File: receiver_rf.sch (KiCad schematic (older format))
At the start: 0 parts

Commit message: Added mixer and LNA
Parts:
- added C? (x2): 22pF, symbol Device:C
- added C?: 22uF, symbol Device:C
- added C?: 100pF, symbol Device:C
- added L?: 10nH, symbol Device:L
- added U?: PMA-63GLN+, symbol own:PMA-63GLN+
- added U?: HMC218BMS8GE, symbol own:HMC218BMS8GE
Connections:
- new net: C?.2, U?.2 (RF_IN)
- new net: C?.1, L?.2, U?.8 (RF_OUT/DC_IN)
- new net: C?.2, U?.8 (RF)
- new net +5V: C?.2, C?.2, L?.1
- new net GND: C?.1, C?.1, U?.13 (GND/Paddle), U?.2 (GND), U?.3 (GND), U?.6 (GND), U?.7 (GND)
- new net IF_OUT: U?.5 (IF)
- new net LO_IN: U?.1 (LO)
- new net RF_IN: C?.1
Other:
- note added: "1.8-6.0GHz\nNF: 1dB\nGain: +26dB\nP1dB: 11dB"
- note added: "Conversion Loss: -7dB\nP1dB: 10dB"
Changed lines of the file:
@@
 $Descr A4 11693 8268
 encoding utf-8
-Sheet 1 6
+Sheet 5 6
 Title ""
 Date ""
@@
 Comment4 ""
 $EndDescr
+Text HLabel 8300 3950 2    100  Input ~ 0
+RF_IN
+Text HLabel 5200 3150 2    100  Input ~ 0
+LO_IN
+Text HLabel 3650 3850 0    100  Output ~ 0
+IF_OUT
+$Comp
+L Device:C C?
+U 1 1 5F8B845C
+P 7850 3950
+F 0 "C?" V 7598 3950 50  0000 C CNN
+F 1 "22pF" V 7689 3950 50  0000 C CNN
+F 2 "" H 7888 3800 50  0001 C CNN
+F 3 "~" H 7850 3950 50  0001 C CNN
+	1    7850 3950
+	0    1    1    0
+$EndComp
+Wire Wire Line
+	7550 3950 7700 3950
+Wire Wire Line
+	8000 3950 8300 3950
+$Comp
+L Device:C C?
+U 1 1 5F8B8D04
+P 5550 3850
+F 0 "C?" V 5298 3850 50  0000 C CNN
+F 1 "22pF" V 5389 3850 50  0000 C CNN
+F 2 "" H 5588 3700 50  0001 C CNN
+F 3 "~" H 5550 3850 50  0001 C CNN
+	1    5550 3850
+	0    1    1    0
+$EndComp
+Wire Wire Line
+	6100 3850 5900 3850
+$Comp
+L Device:L L?
+U 1 1 5F8B94E9
+P 5900 3550
+F 0 "L?" H 5953 3596 50  0000 L CNN
+F 1 "10nH" H 5953 3505 50  0000 L CNN
+F 2 "" H 5900 3550 50  0001 C CNN
+F 3 "~" H 5900 3550 50  0001 C CNN
+	1    5900 3550
+	1    0    0    -1
+$EndComp
+Wire Wire Line
+	5900 3700 5900 3850
+Connection ~ 5900 3850
+Wire Wire Line
+	5900 3850 5700 3850
+Wire Wire Line
+	5900 2650 5900 2850
+$Comp
+L Device:C C?
+U 1 1 5F8BA0F4
+P 6100 2850
+F 0 "C?" V 5848 2850 50  0000 C CNN
+F 1 "22uF" V 5939 2850 50  0000 C CNN
+F 2 "" H 6138 2700 50  0001 C CNN
+F 3 "~" H 6100 2850 50  0001 C CNN
+	1    6100 2850
+	0    1    1    0
+$EndComp
+$Comp
+L Device:C C?
+U 1 1 5F8BA3A2
+P 6100 3250
+F 0 "C?" V 5848 3250 50  0000 C CNN
+F 1 "100pF" V 5939 3250 50  0000 C CNN
+F 2 "" H 6138 3100 50  0001 C CNN
+F 3 "~" H 6100 3250 50  0001 C CNN
+	1    6100 3250
+	0    1    1    0
+$EndComp
+Wire Wire Line
+	5950 2850 5900 2850
+Connection ~ 5900 2850
+Wire Wire Line
+	5900 2850 5900 3250
+Wire Wire Line
+	5950 3250 5900 3250
+Connection ~ 5900 3250
+Wire Wire Line
+	5900 3250 5900 3400
+Wire Wire Line
+	6250 2850 6300 2850
+Wire Wire Line
+	6300 2850 6300 3250
+Wire Wire Line
+	6300 3250 6250 3250
+Wire Wire Line
+	6300 3250 6300 3300
+Connection ~ 6300 3250
+$Comp
+L power:GND #PWR?
+U 1 1 5F8BB071
+P 6300 3300
+F 0 "#PWR?" H 6300 3050 50  0001 C CNN
+F 1 "GND" H 6305 3127 50  0000 C CNN
+F 2 "" H 6300 3300 50  0001 C CNN
+F 3 "" H 6300 3300 50  0001 C CNN
+	1    6300 3300
+	1    0    0    -1
+$EndComp
+$Comp
+L power:GND #PWR?
+U 1 1 5F8BBC9F
+P 6050 4150
+F 0 "#PWR?" H 6050 3900 50  0001 C CNN
+F 1 "GND" H 6055 3977 50  0000 C CNN
+F 2 "" H 6050 4150 50  0001 C CNN
+F 3 "" H 6050 4150 50  0001 C CNN
+	1    6050 4150
+	1    0    0    -1
+$EndComp
+Wire Wire Line
+	6100 4100 6050 4100
+Wire Wire Line
+	6050 4100 6050 4150
+$Comp
+L own:PMA-63GLN+ U?
+U 1 1 5F8BCDE2
+P 6850 3850
+F 0 "U?" H 6825 4165 50  0000 C CNN
+F 1 "PMA-63GLN+" H 6825 4074 50  0000 C CNN
+F 2 "" H 6850 3850 100 0001 C CNN
+F 3 "" H 6850 3850 100 0001 C CNN
+	1    6850 3850
+	1    0    0    -1
+$EndComp
+$Comp
+L power:+5V #PWR?
+U 1 1 5F8BDE8F
+P 5900 2650
+F 0 "#PWR?" H 5900 2500 50  0001 C CNN
+F 1 "+5V" H 5915 2823 50  0000 C CNN
+F 2 "" H 5900 2650 50  0001 C CNN
+F 3 "" H 5900 2650 50  0001 C CNN
+	1    5900 2650
+	1    0    0    -1
+$EndComp
+Wire Wire Line
+	5400 3850 4900 3850
+Wire Wire Line
+	5200 3150 5100 3150
+Wire Wire Line
+	5100 3150 5100 3500
+Wire Wire Line
+	5100 3500 4900 3500
+$Comp
+L own:HMC218BMS8GE U?
+U 1 1 5F8BF630
+P 4350 3650
+F 0 "U?" H 4350 4065 50  0000 C CNN
+F 1 "HMC218BMS8GE" H 4350 3974 50  0000 C CNN
+F 2 "" H 4350 3650 100 0001 C CNN
+F 3 "" H 4350 3650 100 0001 C CNN
+	1    4350 3650
+	1    0    0    -1
+$EndComp
+Wire Wire Line
+	4200 4400 4200 4450
+Wire Wire Line
+	4200 4450 4300 4450
+Wire Wire Line
+	4500 4450 4500 4400
+Wire Wire Line
+	4400 4400 4400 4450
+Connection ~ 4400 4450
+Wire Wire Line
+	4400 4450 4500 4450
+Wire Wire Line
+	4300 4450 4300 4400
+Connection ~ 4300 4450
+Wire Wire Line
+	4300 4450 4400 4450
+$Comp
+L power:GND #PWR?
+U 1 1 5F8C05DA
+P 4500 4500
+F 0 "#PWR?" H 4500 4250 50  0001 C CNN
+F 1 "GND" H 4505 4327 50  0000 C CNN
+F 2 "" H 4500 4500 50  0001 C CNN
+F 3 "" H 4500 4500 50  0001 C CNN
+	1    4500 4500
+	1    0    0    -1
+$EndComp
+Wire Wire Line
+	4500 4450 4500 4500
+Connection ~ 4500 4450
+Wire Wire Line
+	3800 3850 3650 3850
+Text Notes 7000 4600 0    50   ~ 0
+1.8-6.0GHz\nNF: 1dB\nGain: +26dB\nP1dB: 11dB
+Text Notes 4650 4550 0    50   ~ 0
+Conversion Loss: -7dB\nP1dB: 10dB
 $EndSCHEMATC

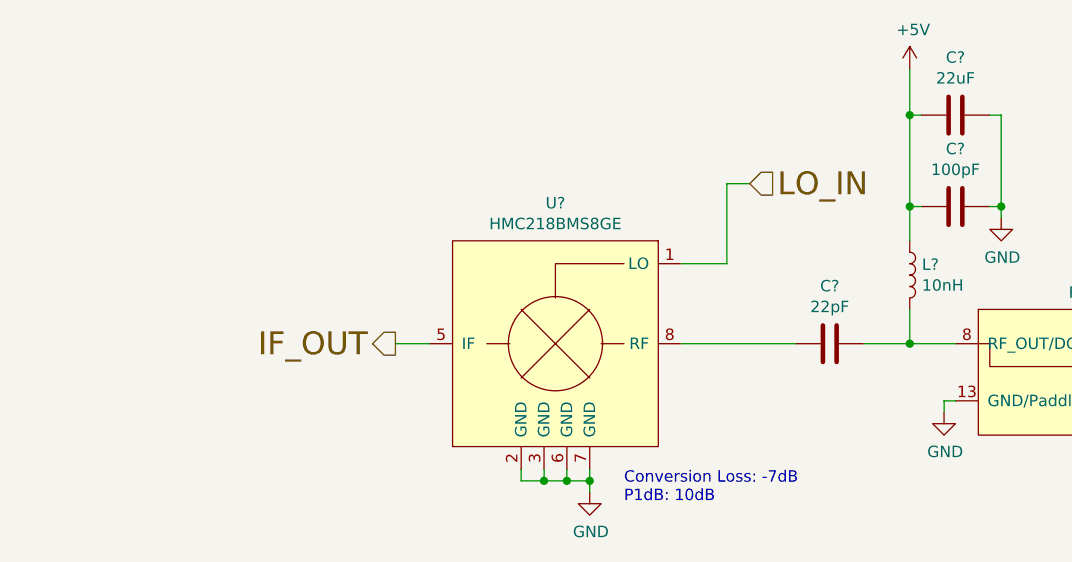
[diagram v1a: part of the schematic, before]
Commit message: Architecture of IF
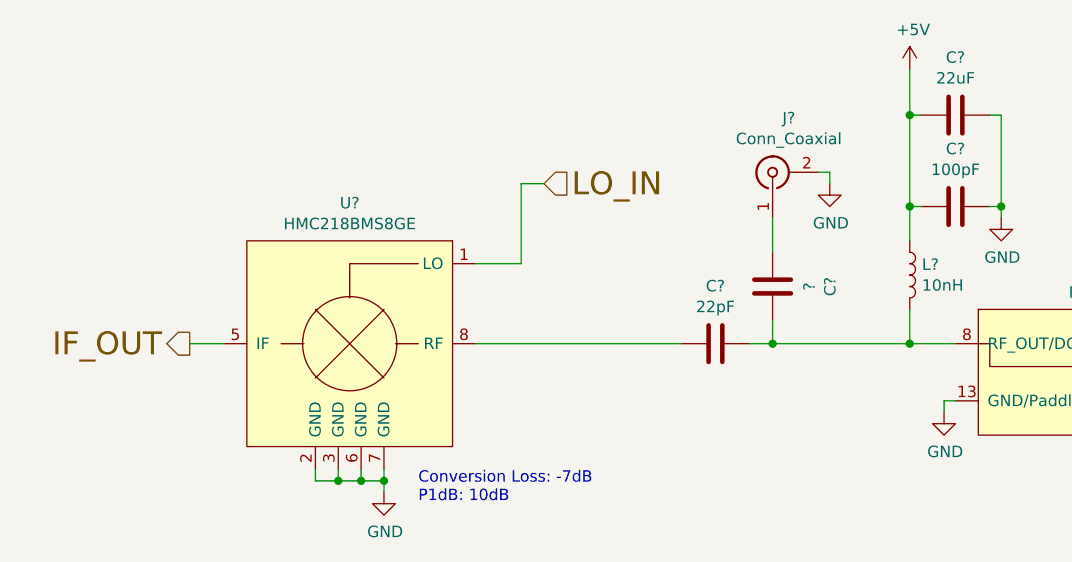
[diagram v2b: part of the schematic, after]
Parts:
- added C?: ?, symbol Device:C
- added J?: Conn_Coaxial, symbol Connector:Conn_Coaxial
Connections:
- net GND: now also J?.2 (Ext)
- net at C?.1, L?.2, U?.8 (RF_OUT/DC_IN): now also C?.1
- new net: C?.2, J?.1 (In)
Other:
- moved on the sheet: C?, U?
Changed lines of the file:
@@
 Text HLabel 8300 3950 2    100  Input ~ 0
 RF_IN
-Text HLabel 5200 3150 2    100  Input ~ 0
+Text HLabel 4300 3150 2    100  Input ~ 0
 LO_IN
-Text HLabel 3650 3850 0    100  Output ~ 0
+Text HLabel 2750 3850 0    100  Output ~ 0
 IF_OUT
 $Comp
@@
 L Device:C C?
 U 1 1 5F8B8D04
-P 5550 3850
-F 0 "C?" V 5298 3850 50  0000 C CNN
-F 1 "22pF" V 5389 3850 50  0000 C CNN
-F 2 "" H 5588 3700 50  0001 C CNN
-F 3 "~" H 5550 3850 50  0001 C CNN
-	1    5550 3850
+P 5050 3850
+F 0 "C?" V 4798 3850 50  0000 C CNN
+F 1 "22pF" V 4889 3850 50  0000 C CNN
+F 2 "" H 5088 3700 50  0001 C CNN
+F 3 "~" H 5050 3850 50  0001 C CNN
+	1    5050 3850
 	0    1    1    0
 $EndComp
@@
 Connection ~ 5900 3850
 Wire Wire Line
-	5900 3850 5700 3850
+	5900 3850 5300 3850
 Wire Wire Line
 	5900 2650 5900 2850
@@
 $EndComp
 Wire Wire Line
-	5400 3850 4900 3850
-Wire Wire Line
-	5200 3150 5100 3150
-Wire Wire Line
-	5100 3150 5100 3500
-Wire Wire Line
-	5100 3500 4900 3500
+	4300 3150 4200 3150
+Wire Wire Line
+	4200 3150 4200 3500
+Wire Wire Line
+	4200 3500 4000 3500
 $Comp
 L own:HMC218BMS8GE U?
 U 1 1 5F8BF630
-P 4350 3650
-F 0 "U?" H 4350 4065 50  0000 C CNN
-F 1 "HMC218BMS8GE" H 4350 3974 50  0000 C CNN
-F 2 "" H 4350 3650 100 0001 C CNN
-F 3 "" H 4350 3650 100 0001 C CNN
-	1    4350 3650
-	1    0    0    -1
-$EndComp
-Wire Wire Line
-	4200 4400 4200 4450
-Wire Wire Line
-	4200 4450 4300 4450
-Wire Wire Line
-	4500 4450 4500 4400
-Wire Wire Line
-	4400 4400 4400 4450
-Connection ~ 4400 4450
-Wire Wire Line
-	4400 4450 4500 4450
-Wire Wire Line
-	4300 4450 4300 4400
-Connection ~ 4300 4450
-Wire Wire Line
-	4300 4450 4400 4450
+P 3450 3650
+F 0 "U?" H 3450 4065 50  0000 C CNN
+F 1 "HMC218BMS8GE" H 3450 3974 50  0000 C CNN
+F 2 "" H 3450 3650 100 0001 C CNN
+F 3 "" H 3450 3650 100 0001 C CNN
+	1    3450 3650
+	1    0    0    -1
+$EndComp
+Wire Wire Line
+	3300 4400 3300 4450
+Wire Wire Line
+	3300 4450 3400 4450
+Wire Wire Line
+	3600 4450 3600 4400
+Wire Wire Line
+	3500 4400 3500 4450
+Connection ~ 3500 4450
+Wire Wire Line
+	3500 4450 3600 4450
+Wire Wire Line
+	3400 4450 3400 4400
+Connection ~ 3400 4450
+Wire Wire Line
+	3400 4450 3500 4450
 $Comp
 L power:GND #PWR?
 U 1 1 5F8C05DA
-P 4500 4500
-F 0 "#PWR?" H 4500 4250 50  0001 C CNN
-F 1 "GND" H 4505 4327 50  0000 C CNN
-F 2 "" H 4500 4500 50  0001 C CNN
-F 3 "" H 4500 4500 50  0001 C CNN
-	1    4500 4500
-	1    0    0    -1
-$EndComp
-Wire Wire Line
-	4500 4450 4500 4500
-Connection ~ 4500 4450
-Wire Wire Line
-	3800 3850 3650 3850
+P 3600 4500
+F 0 "#PWR?" H 3600 4250 50  0001 C CNN
+F 1 "GND" H 3605 4327 50  0000 C CNN
+F 2 "" H 3600 4500 50  0001 C CNN
+F 3 "" H 3600 4500 50  0001 C CNN
+	1    3600 4500
+	1    0    0    -1
+$EndComp
+Wire Wire Line
+	3600 4450 3600 4500
+Connection ~ 3600 4450
+Wire Wire Line
+	2900 3850 2750 3850
 Text Notes 7000 4600 0    50   ~ 0
 1.8-6.0GHz\nNF: 1dB\nGain: +26dB\nP1dB: 11dB
-Text Notes 4650 4550 0    50   ~ 0
+Text Notes 3750 4550 0    50   ~ 0
 Conversion Loss: -7dB\nP1dB: 10dB
+Wire Wire Line
+	4000 3850 4900 3850
+$Comp
+L Device:C C?
+U 1 1 5FA1A18D
+P 5300 3600
+F 0 "C?" V 5048 3600 50  0000 C CNN
+F 1 "?" V 5139 3600 50  0000 C CNN
+F 2 "" H 5338 3450 50  0001 C CNN
+F 3 "~" H 5300 3600 50  0001 C CNN
+	1    5300 3600
+	-1   0    0    1
+$EndComp
+Wire Wire Line
+	5300 3750 5300 3850
+Connection ~ 5300 3850
+Wire Wire Line
+	5300 3850 5200 3850
+$Comp
+L Connector:Conn_Coaxial J?
+U 1 1 5FA1B39E
+P 5300 3100
+F 0 "J?" V 5537 3029 50  0000 C CNN
+F 1 "Conn_Coaxial" V 5446 3029 50  0000 C CNN
+F 2 "" H 5300 3100 50  0001 C CNN
+F 3 " ~" H 5300 3100 50  0001 C CNN
+	1    5300 3100
+	0    -1   -1   0
+$EndComp
+Wire Wire Line
+	5300 3300 5300 3450
+$Comp
+L power:GND #PWR?
+U 1 1 5FA1CDDA
+P 5550 3150
+F 0 "#PWR?" H 5550 2900 50  0001 C CNN
+F 1 "GND" H 5555 2977 50  0000 C CNN
+F 2 "" H 5550 3150 50  0001 C CNN
+F 3 "" H 5550 3150 50  0001 C CNN
+	1    5550 3150
+	1    0    0    -1
+$EndComp
+Wire Wire Line
+	5500 3100 5550 3100
+Wire Wire Line
+	5550 3100 5550 3150
 $EndSCHEMATC

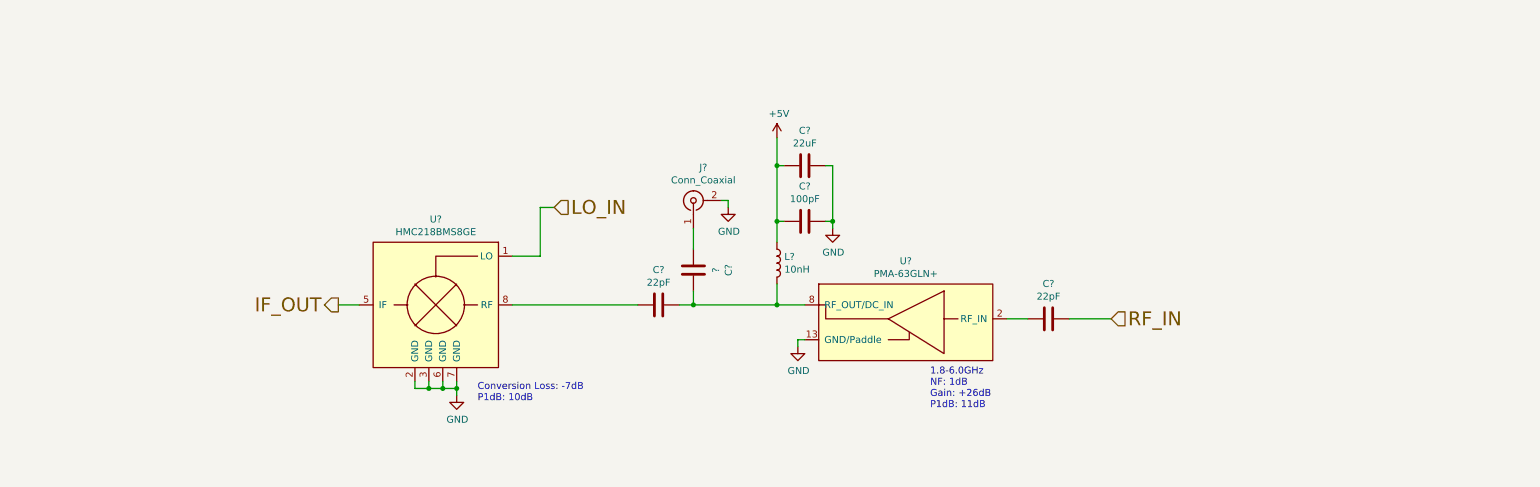
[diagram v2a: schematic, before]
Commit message: Finished IF
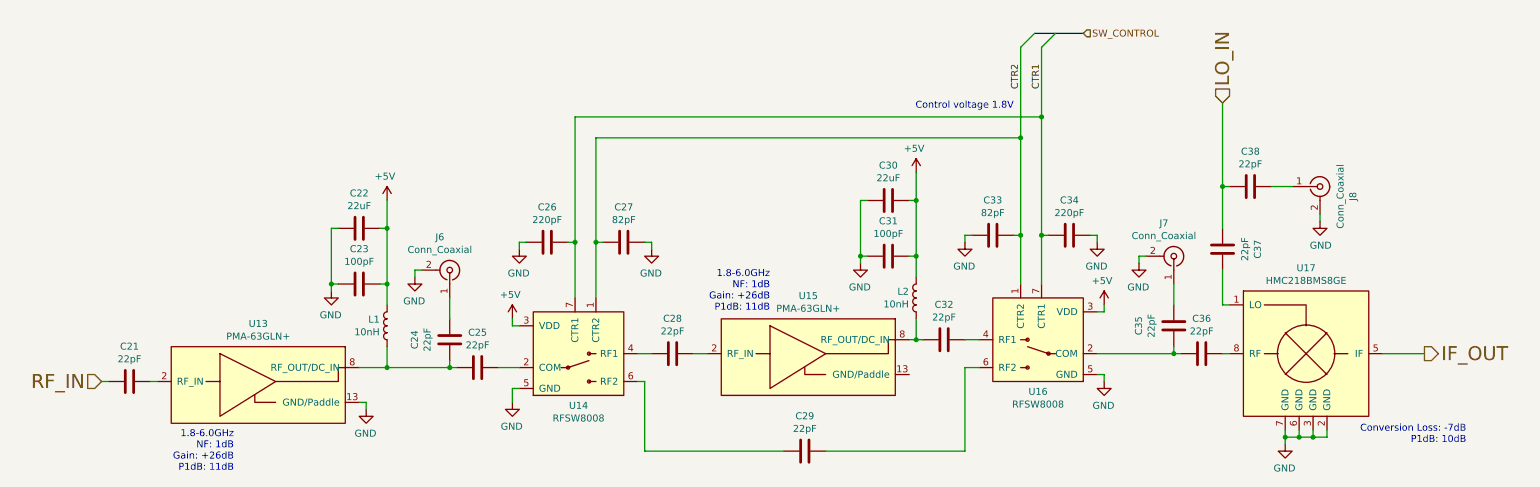
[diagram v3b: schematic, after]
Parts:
- added C25, C28, C29, C32, C35, C37, C38: 22pF, Capacitor_SMD:C_0402_1005Metric_Pad0.74x0.62mm_HandSolder, symbol Device:C
- added C26, C34: 220pF, Capacitor_SMD:C_0603_1608Metric_Pad1.08x0.95mm_HandSolder, symbol Device:C
- added C27, C33: 82pF, Capacitor_SMD:C_0603_1608Metric_Pad1.08x0.95mm_HandSolder, symbol Device:C
- added C30: 22uF, Capacitor_SMD:C_0603_1608Metric_Pad1.08x0.95mm_HandSolder, symbol Device:C
- added C31: 100pF, Capacitor_SMD:C_0603_1608Metric_Pad1.08x0.95mm_HandSolder, symbol Device:C
- added J7, J8: Conn_Coaxial, symbol Connector:Conn_Coaxial
- added L2: 10nH, Inductor_SMD:L_0402_1005Metric_Pad0.77x0.64mm_HandSolder, symbol Device:L
- added U14, U16: RFSW8008, symbol own:RFSW8008
- added U15: PMA-63GLN+, Package_DFN_QFN:QFN-12-1EP_3x3mm_P0.51mm_EP1.45x1.45mm, symbol own:PMA-63GLN+
- C21, C36: renamed from C?; footprint (none) -> Capacitor_SMD:C_0402_1005Metric_Pad0.74x0.62mm_HandSolder
- C22, C23: renamed from C?; footprint (none) -> Capacitor_SMD:C_0603_1608Metric_Pad1.08x0.95mm_HandSolder
- C24: renamed from C?; value ? -> 22pF; footprint (none) -> Capacitor_SMD:C_0402_1005Metric_Pad0.74x0.62mm_HandSolder
- L1: renamed from L?; footprint (none) -> Inductor_SMD:L_0402_1005Metric_Pad0.77x0.64mm_HandSolder
- U13: renamed from U?; footprint (none) -> Package_DFN_QFN:QFN-12-1EP_3x3mm_P0.51mm_EP1.45x1.45mm
- U17: renamed from U?; footprint (none) -> Package_SO:MSOP-8-1EP_3x3mm_P0.65mm_EP1.73x1.85mm
- gave numbers to parts that had none: 1
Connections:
- net +5V: now also C30.2, C31.2, L2.1, U14.3 (VDD), U16.3 (VDD)
- net GND: now also C26.1, C27.2, C30.1, C31.1, C33.1, C34.2, J7.2 (Ext), J8.2 (Ext), U14.5 (GND), U16.5 (GND)
- net LO_IN: now also C37.1, C38.1; no longer U17.1 (LO)
- net at C24.1, L1.2, U13.8 (RF_OUT/DC_IN): now also C25.1; no longer C36.1
- new net: C35.1, C36.1, U16.2 (COM)
- new net: C37.2, U17.1 (LO)
- new net: C25.2, U14.2 (COM)
- new net: C28.1, U14.4 (RF1)
- new net: C29.1, U14.6 (RF2)
- new net: C28.2, U15.2 (RF_IN)
- new net: C32.1, L2.2, U15.8 (RF_OUT/DC_IN)
- new net: C32.2, U16.4 (RF1)
- new net: C29.2, U16.6 (RF2)
- new net: C35.2, J7.1 (In)
- new net: C38.2, J8.1 (In)
- new net CTR1: C26.2, C34.1, U14.7 (CTR1), U16.7 (CTR1)
- new net CTR2: C27.1, C33.2, U14.1 (CTR2), U16.1 (CTR2)
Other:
- note added: "Control voltage 1.8V"
- moved on the sheet: C21, C22, C23, C24, C36, J6, L1, U13, U17
